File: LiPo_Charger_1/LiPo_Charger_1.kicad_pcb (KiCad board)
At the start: 2 copper layers, 42 x 16 mm, 23 parts, among them IC1 FS312F-G, J1 USB_B_Micro, J2 Conn_01x02_Female, J3 USB_B_Micro, Q1 FS8205, SW1 SW_DIP_x01, U1 TP4056_[C16581], U2 MT3608

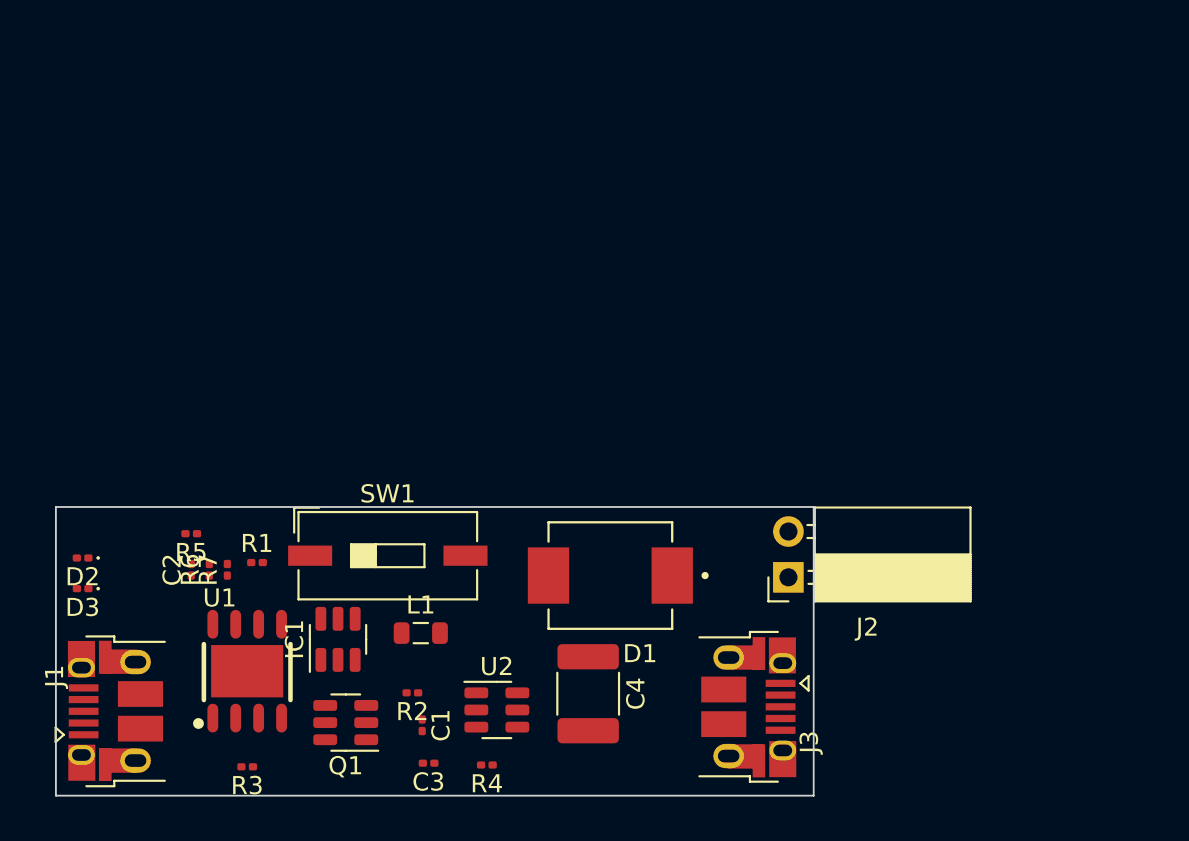
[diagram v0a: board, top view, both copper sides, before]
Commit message: 09/30/22
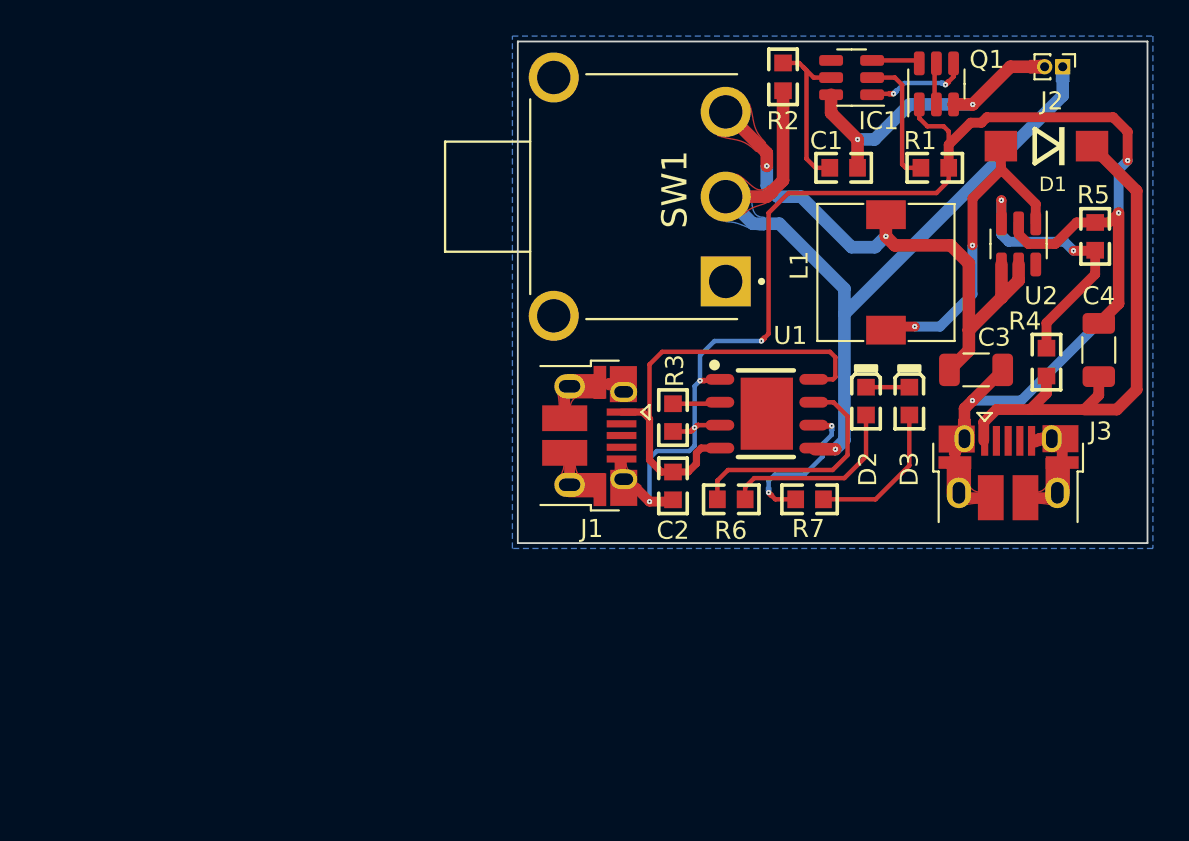
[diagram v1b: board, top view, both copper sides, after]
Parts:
- C1, C2: footprint Capacitor_SMD:C_0201_0603Metric -> lc_lib:0603_R
- C3: value 10u -> 22uF; footprint Capacitor_SMD:C_0201_0603Metric -> Capacitor_SMD:C_1206_3216Metric
- C4: footprint Capacitor_SMD:C_1812_4532Metric -> Capacitor_SMD:C_1206_3216Metric
- D1: value SS34_V7G -> SS34_mdd; footprint 403_charger:DIOM6859X262N -> 403_charger:SS34_mdd
- D2, D3: footprint LED_SMD:LED_0201_0603Metric -> lc_lib:0603_LED_S1
- J2: footprint Connector_PinSocket_2.54mm:PinSocket_1x02_P2.54mm_Horizontal -> Connector_PinHeader_1.00mm:PinHeader_1x02_P1.00mm_Vertical
- L1: footprint Inductor_SMD:L_0805_2012Metric -> 403_charger:75_75_4
- R1, R2, R3, R4, R5, R6, R7: footprint Resistor_SMD:R_0201_0603Metric -> lc_lib:0603_R
- SW1: footprint Button_Switch_SMD:SW_DIP_SPSTx01_Slide_9.78x4.72mm_W8.61mm_P2.54mm -> 403_charger:SW_500SSP3S1M6QEA
- moved R5 52.7 mm to (175.6, 66.0), turned to 90 degrees
- moved Q1 48.2 mm to (166.8, 57.5), turned to 90 degrees
- moved D3 47.0 mm to (165.3, 75.1), turned to -90 degrees
- moved D2 44.3 mm to (162.9, 75.1), turned to -90 degrees
- moved R1 43.5 mm to (166.7, 62.2), turned to 180 degrees
- moved IC1 42.2 mm to (162.1, 57.2), turned to 180 degrees
- moved R2 39.8 mm to (158.3, 57.2), turned to -90 degrees
- moved U2 38.8 mm to (171.4, 66.4), turned to -90 degrees
- moved C1 38.7 mm to (161.7, 62.2), turned to 0 degrees
- moved R4 38.2 mm to (172.9, 73.0), turned to 90 degrees
- moved C3 37.4 mm to (169.0, 73.4), turned to 0 degrees
- moved C4 34.1 mm to (175.8, 72.3), turned to 90 degrees
- moved L1 33.9 mm to (168.0, 71.8), turned to 90 degrees
- moved D1 33.9 mm to (172.9, 61.0)
- moved R7 32.5 mm to (159.8, 80.6), turned to 0 degrees
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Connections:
- SW1 pad 1: /BAT+ -> unconnected-(SW1-Pad1)
- SW1 pad 2: Net-(C3-Pad1) -> /BAT+
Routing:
- net GND: track 0.00 -> 109.5 mm, vias 0 -> 7
- net /BAT+: track 0.00 -> 46.2 mm, vias 0 -> 1
- net Net-(C3-Pad1): track 0.00 -> 32.7 mm, vias 0 -> 2
- net /5V: track 0.00 -> 29.2 mm
- net /VBUS: track 0.00 -> 25.1 mm
- net Net-(D1-PadA): track 0.00 -> 18.4 mm, vias 0 -> 2
- net /BAT-: track 0.00 -> 17.8 mm, vias 0 -> 2
- net Net-(R4-Pad2): track 0.00 -> 15.3 mm, vias 0 -> 2
- net Net-(R6-Pad1): track 0.00 -> 13.2 mm
- net Net-(D2-Pad1): track 0.00 -> 10.4 mm
- net Net-(C1-Pad1): track 0.00 -> 9.61 mm
- net Net-(R7-Pad1): track 0.00 -> 8.79 mm, vias 0 -> 2
- net Net-(D3-Pad1): track 0.00 -> 8.34 mm
- net Net-(IC1-Pad2): track 0.00 -> 7.35 mm
- net /OD: track 0.00 -> 5.75 mm, vias 0 -> 2
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- added copper zone on B.Cu, net GND
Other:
- board size 42 x 16 mm -> 34.9 x 27.8 mm
